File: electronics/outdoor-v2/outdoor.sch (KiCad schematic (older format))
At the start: 9 parts, among them J1 TX433MHz, U1 ATtiny85V-10PU, U2 DS18B20

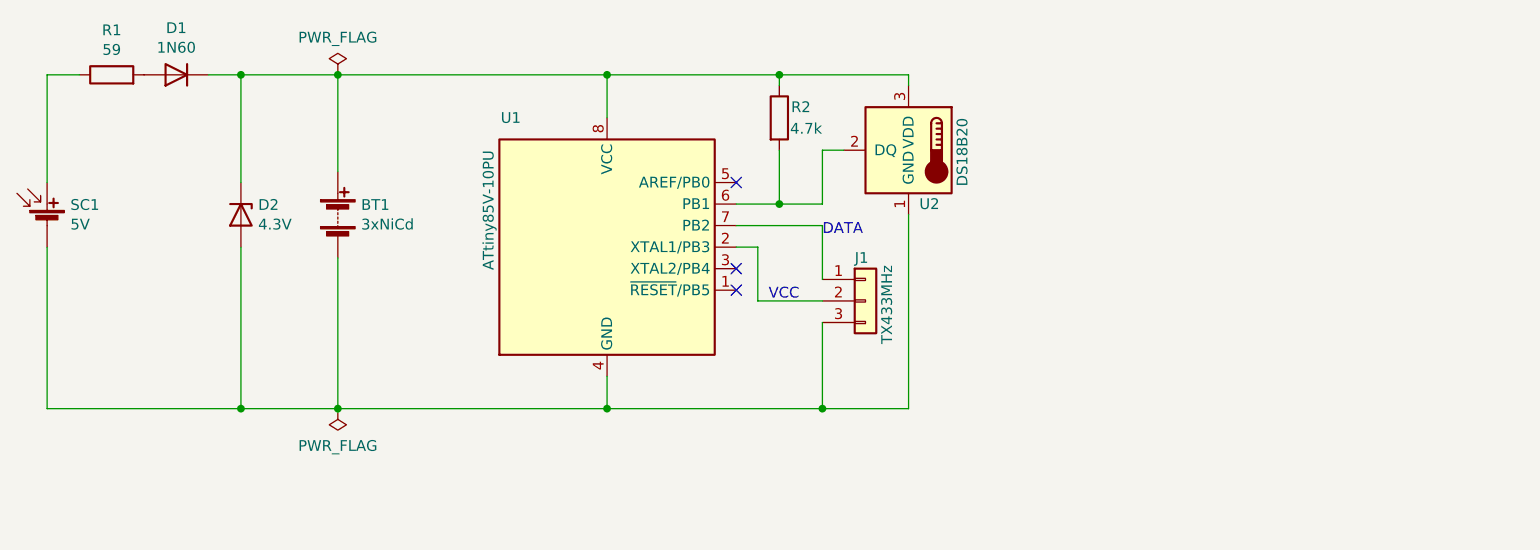
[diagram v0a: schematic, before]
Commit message: outdoor unit revision WIP
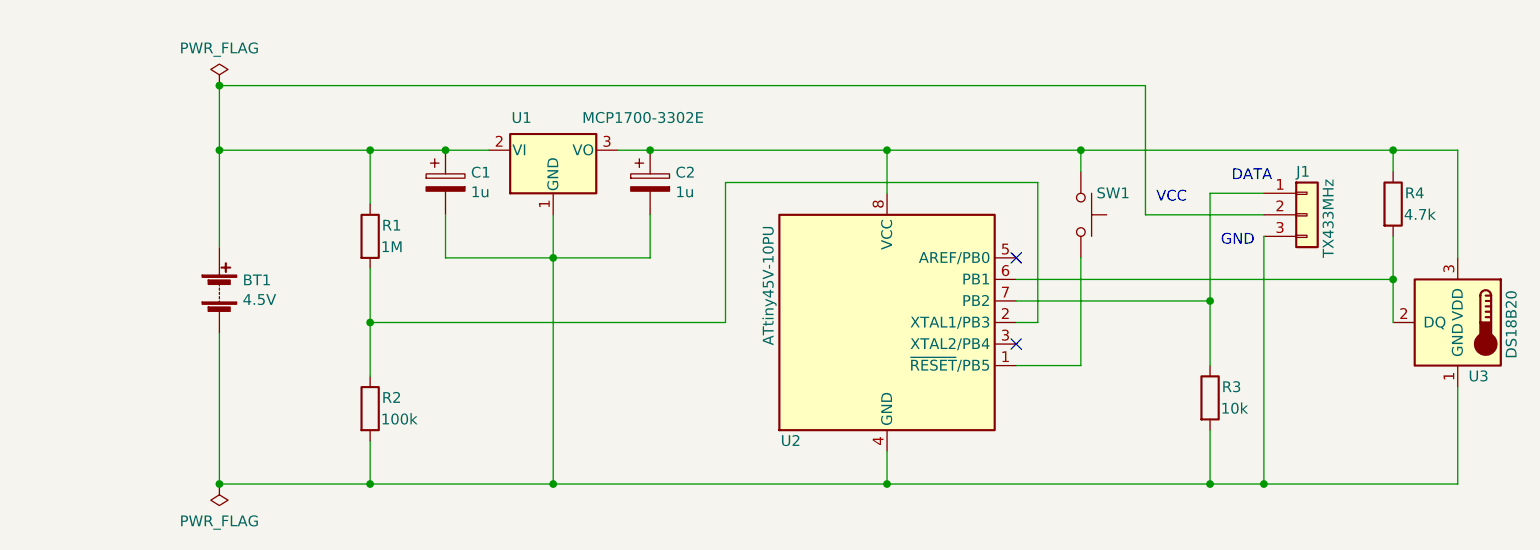
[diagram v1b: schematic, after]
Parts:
- removed D1: 1N60, Diode_THT:D_DO-35_SOD27_P10.16mm_Horizontal, symbol Device:D
- removed D2: 4.3V, Diode_THT:D_DO-35_SOD27_P10.16mm_Horizontal, symbol Device:D_Zener
- removed SC1: 5V, Connector_PinHeader_2.54mm:PinHeader_1x02_P2.54mm_Vertical, symbol Device:Solar_Cell
- added C1, C2: 1u, Capacitor_THT:C_Rect_L7.0mm_W2.5mm_P5.00mm, symbol Device:CP
- added R2: 100k, Resistor_THT:R_Axial_DIN0207_L6.3mm_D2.5mm_P10.16mm_Horizontal, symbol Device:R
- added R3: 10k, Resistor_THT:R_Axial_DIN0207_L6.3mm_D2.5mm_P10.16mm_Horizontal, symbol Device:R
- added SW1: SW_Push, Button_Switch_THT:SW_PUSH_6mm, symbol Switch:SW_Push
- added U1: MCP1700-3302E, Package_TO_SOT_THT:TO-92_Inline_Wide, symbol Regulator_Linear:MCP1700-3302E_TO92
- BT1: value 3xNiCd -> 4.5V; footprint CustomParts:NiCd-Small -> Connector_PinHeader_2.54mm:PinHeader_1x02_P2.54mm_Vertical
- R1: value 59 -> 1M
- U2: renamed from U1; value ATtiny85V-10PU -> ATtiny45V-10PU
- renumbered R2 to R4, U2 to U3
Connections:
- net at R4.1, U2.8 (VCC), U3.3 (VDD): now also C2.1, SW1.1, U1.3 (VO); no longer BT1.1 (+)
- net at BT1.2 (-), J1.3 (Pin_3), U2.4 (GND)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: now also C1.2, C2.2, R2.2, R3.2, U1.1 (GND)
- net at R1.1: now also BT1.1 (+), J1.2 (Pin_2), C1.1, U1.2 (VI)
- net at R1.2: now also U2.2 (XTAL1/PB3), R2.1
- net at U2.1 (~RESET~/PB5): now also SW1.2
- net at J1.1 (Pin_1), U2.7 (PB2): now also R3.1
- no-connect marks 3 -> 2
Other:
- note added: "GND"
- moved on the sheet: J1, R4, U2, U3
